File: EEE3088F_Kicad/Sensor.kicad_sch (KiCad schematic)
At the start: 20 parts, among them IC1 AS5600-ASOT, U5 DRV5032FCDBZR, U6 MCP9700T-E/TT

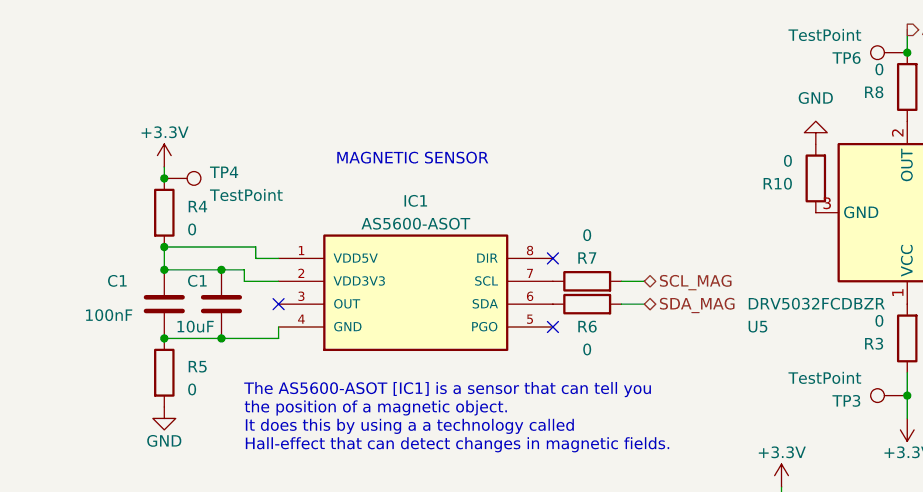
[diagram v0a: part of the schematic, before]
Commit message: Changes made.
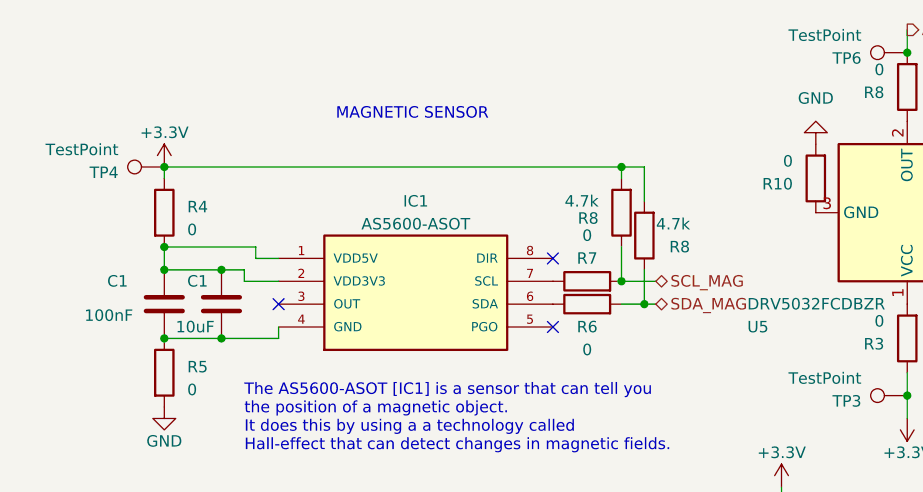
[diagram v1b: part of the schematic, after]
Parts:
- added R8 (x2): 4.7k, symbol Device:R
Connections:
- net +3.3V: now also R8.2, R8.2
- net SCL_MAG: now also R8.1
- net SDA_MAG: now also R8.1
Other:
- moved on the sheet: TP4
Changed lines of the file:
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@@
   (junction (at 46.99 86.36) (diameter 0) (color 0 0 0 0)
   )
+  (junction (at 91.44 74.93) (diameter 0) (color 0 0 0 0)
+  )
   (junction (at 40.64 93.98) (diameter 0) (color 0 0 0 0)
   )
+  (junction (at 91.44 87.63) (diameter 0) (color 0 0 0 0)
+  )
   (junction (at 109.22 113.03) (diameter 0) (color 0 0 0 0)
   )
   (junction (at 121.92 129.54) (diameter 0) (color 0 0 0 0)
   )
+  (junction (at 93.98 90.17) (diameter 0) (color 0 0 0 0)
+  )
   (junction (at 123.19 100.33) (diameter 0) (color 0 0 0 0)
   )
-  (junction (at 40.64 76.2) (diameter 0) (color 0 0 0 0)
-  )
   (junction (at 123.19 62.23) (diameter 0) (color 0 0 0 0)
+  )
+  (junction (at 40.64 74.93) (diameter 0) (color 0 0 0 0)
   )
   (junction (at 40.64 83.82) (diameter 0) (color 0 0 0 0)
@@
     (stroke (width 0) (type default))
   )
+  (wire (pts (xy 91.44 90.17) (xy 93.98 90.17))
+    (stroke (width 0) (type default))
+  )
+  (wire (pts (xy 93.98 78.74) (xy 93.98 74.93))
+    (stroke (width 0) (type default))
+  )
   (wire (pts (xy 53.34 93.98) (xy 53.34 92.71))
     (stroke (width 0) (type default))
@@
     (stroke (width 0) (type default))
   )
-  (wire (pts (xy 91.44 90.17) (xy 93.98 90.17))
-    (stroke (width 0) (type default))
-  )
   (wire (pts (xy 40.64 74.93) (xy 40.64 76.2))
     (stroke (width 0) (type default))
   )
+  (wire (pts (xy 91.44 74.93) (xy 93.98 74.93))
+    (stroke (width 0) (type default))
+  )
+  (wire (pts (xy 93.98 90.17) (xy 95.25 90.17))
+    (stroke (width 0) (type default))
+  )
   (wire (pts (xy 123.19 100.33) (xy 123.19 97.79))
     (stroke (width 0) (type default))
@@
     (stroke (width 0) (type default))
   )
-  (wire (pts (xy 91.44 87.63) (xy 93.98 87.63))
+  (wire (pts (xy 91.44 74.93) (xy 91.44 76.2))
+    (stroke (width 0) (type default))
+  )
+  (wire (pts (xy 91.44 87.63) (xy 95.25 87.63))
     (stroke (width 0) (type default))
   )
@@
     (stroke (width 0) (type default))
   )
+  (wire (pts (xy 91.44 83.82) (xy 91.44 87.63))
+    (stroke (width 0) (type default))
+  )
   (wire (pts (xy 116.84 129.54) (xy 121.92 129.54))
     (stroke (width 0) (type default))
@@
     (stroke (width 0) (type default))
   )
+  (wire (pts (xy 93.98 86.36) (xy 93.98 90.17))
+    (stroke (width 0) (type default))
+  )
   (wire (pts (xy 40.64 93.98) (xy 46.99 93.98))
     (stroke (width 0) (type default))
   )
+  (wire (pts (xy 40.64 74.93) (xy 91.44 74.93))
+    (stroke (width 0) (type default))
+  )
   (wire (pts (xy 49.53 87.63) (xy 53.34 87.63))
     (stroke (width 0) (type default))
   )
-  (text "MAGNETIC SENSOR" (at 59.69 74.93 0)
+  (text "MAGNETIC SENSOR" (at 59.69 69.85 0)
     (effects (font (size 1.27 1.27)) (justify left bottom))
   )
@@
     (effects (font (size 1.27 1.27)) (justify left))
   )
-  (hierarchical_label "SDA_MAG" (shape bidirectional) (at 93.98 90.17 0) (fields_autoplaced)
+  (hierarchical_label "SDA_MAG" (shape bidirectional) (at 95.25 90.17 0) (fields_autoplaced)
     (effects (font (size 1.27 1.27)) (justify left))
   )
@@
     (effects (font (size 1.27 1.27)) (justify left))
   )
-  (hierarchical_label "SCL_MAG" (shape bidirectional) (at 93.98 87.63 0) (fields_autoplaced)
+  (hierarchical_label "SCL_MAG" (shape bidirectional) (at 95.25 87.63 0) (fields_autoplaced)
     (effects (font (size 1.27 1.27)) (justify left))
   )
@@
     )
   )
-  (symbol (lib_id "Connector:TestPoint") (at 40.64 76.2 270) (unit 1)
-    (in_bom yes) (on_board yes) (dnp no) (fields_autoplaced)
-    (property "Reference" "TP4" (at 45.72 75.565 90)
-      (effects (font (size 1.27 1.27)) (justify left))
-    )
-    (property "Value" "TestPoint" (at 45.72 78.105 90)
-      (effects (font (size 1.27 1.27)) (justify left))
-    )
-    (property "Footprint" "" (at 40.64 81.28 0)
-      (effects (font (size 1.27 1.27)) hide)
-    )
-    (property "Datasheet" "~" (at 40.64 81.28 0)
+  (symbol (lib_id "Connector:TestPoint") (at 40.64 74.93 90) (unit 1)
+    (in_bom yes) (on_board yes) (dnp no)
+    (property "Reference" "TP4" (at 35.56 75.565 90)
+      (effects (font (size 1.27 1.27)) (justify left))
+    )
+    (property "Value" "TestPoint" (at 35.56 73.025 90)
+      (effects (font (size 1.27 1.27)) (justify left))
+    )
+    (property "Footprint" "" (at 40.64 69.85 0)
+      (effects (font (size 1.27 1.27)) hide)
+    )
+    (property "Datasheet" "~" (at 40.64 69.85 0)
       (effects (font (size 1.27 1.27)) hide)
     )
@@
     )
   )
+  (symbol (lib_id "Device:R") (at 93.98 82.55 180) (unit 1)
+    (in_bom yes) (on_board yes) (dnp no)
+    (property "Reference" "R8" (at 99.06 83.82 0)
+      (effects (font (size 1.27 1.27)) (justify left))
+    )
+    (property "Value" "4.7k" (at 99.06 81.28 0)
+      (effects (font (size 1.27 1.27)) (justify left))
+    )
+    (property "Footprint" "" (at 95.758 82.55 90)
+      (effects (font (size 1.27 1.27)) hide)
+    )
+    (property "Datasheet" "~" (at 93.98 82.55 0)
+      (effects (font (size 1.27 1.27)) hide)
+    )
+    (pin "1")
+    (pin "2")
+    (instances
+      (project "EEE3088F_Kicad"
+        (path "/6f03c876-746d-4bbb-b455-2f8bb16ffc56/d0e1c216-fa44-4b75-912a-656721c3051d"
+          (reference "R8") (unit 1)
+        )
+      )
+      (project "Sensor"
+        (path "/bd322b28-93df-417b-951b-ff2210130ef6"
+          (reference "R41") (unit 1)
+        )
+      )
+    )
+  )
   (symbol (lib_id "power:+3.3V") (at 109.22 110.49 0) (unit 1)
     (in_bom yes) (on_board yes) (dnp no) (fields_autoplaced)
@@
         )
       )
+    )
+  )
+  (symbol (lib_id "Device:R") (at 91.44 80.01 180) (unit 1)
+    (in_bom yes) (on_board yes) (dnp no)
+    (property "Reference" "R8" (at 88.9 80.645 0)
+      (effects (font (size 1.27 1.27)) (justify left))
+    )
+    (property "Value" "4.7k" (at 88.9 78.74 0)
+      (effects (font (size 1.27 1.27)) (justify left))
+    )
+    (property "Footprint" "" (at 93.218 80.01 90)
+      (effects (font (size 1.27 1.27)) hide)
+    )
+    (property "Datasheet" "~" (at 91.44 80.01 0)
+      (effects (font (size 1.27 1.27)) hide)
+    )
+    (pin "1")
+    (pin "2")
+    (instances
+      (project "EEE3088F_Kicad"
+        (path "/6f03c876-746d-4bbb-b455-2f8bb16ffc56/d0e1c216-fa44-4b75-912a-656721c3051d"
+          (reference "R8") (unit 1)
+        )
+      )
+      (project "Sensor"
+        (path "/bd322b28-93df-417b-951b-ff2210130ef6"
+          (reference "R40") (unit 1)
+        )
+      )
